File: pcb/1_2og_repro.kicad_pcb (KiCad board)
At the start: 2 copper layers, 347.1 x 119.3 mm, 226 parts, among them J1 Pico EzMate, J2 548190519, J3 RAW, J4 S3B, Q1 2N7002, SW1 MX_SW_solder, SW10 MX_SW_solder, SW11 MX_SW_solder, SW12 MX_SW_solder, SW13 MX_SW_solder, SW14 MX_SW_solder, SW15 MX_SW_solder, SW16 MX_SW_solder, SW17 MX_SW_solder, SW18 MX_SW_solder, SW19 MX_SW_solder, SW2 MX_SW_solder, SW20 MX_SW_solder, SW21 MX_SW_solder, SW22 MX_SW_solder, SW23 MX_SW_solder, SW24 MX_SW_solder, SW25 MX_SW_solder, SW26 MX_SW_solder, SW27 MX_SW_solder, SW28 MX_SW_solder, SW29 MX_SW_solder, SW3 MX_SW_solder, SW30 MX_SW_solder, SW31 MX_SW_solder, SW32 MX_SW_solder, SW33 MX_SW_solder, SW34 MX_SW_solder, SW35 MX_SW_solder, SW36 MX_SW_solder, SW37 MX_SW_solder, SW38 MX_SW_solder, SW39 MX_SW_solder, SW4 MX_SW_solder, SW40 MX_SW_solder, SW41 MX_SW_solder, SW42 MX_SW_solder, SW43 MX_SW_solder, SW44 MX_SW_solder, SW45 MX_SW_solder, SW46 MX_SW_solder, SW47 MX_SW_solder, SW48 MX_SW_solder, SW49 MX_SW_solder, SW5 MX_SW_solder, SW50 MX_SW_solder, SW51 MX_SW_solder, SW52 MX_SW_solder, SW53 MX_SW_solder, SW54 MX_SW_solder, SW55 MX_SW_solder, SW56 MX_SW_solder, SW57 MX_SW_solder, SW58 MX_SW_solder, SW59 MX_SW_solder, SW6 MX_SW_solder, SW60 MX_SW_solder, SW61 MX_SW_solder, SW62 MX_SW_solder, SW63 MX_SW_solder, SW64 MX_SW_solder, SW65 MX_SW_solder, SW66 MX_SW_solder, SW67 MX_SW_solder, SW68 MX_SW_solder, SW69 MX_SW_solder, SW7 MX_SW_solder, SW70 MX_SW_solder, SW71 MX_SW_solder, SW72 MX_SW_solder, SW73 MX_SW_solder, SW74 MX_SW_solder, SW75 MX_SW_solder, SW76 MX_SW_solder, SW77 MX_SW_solder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

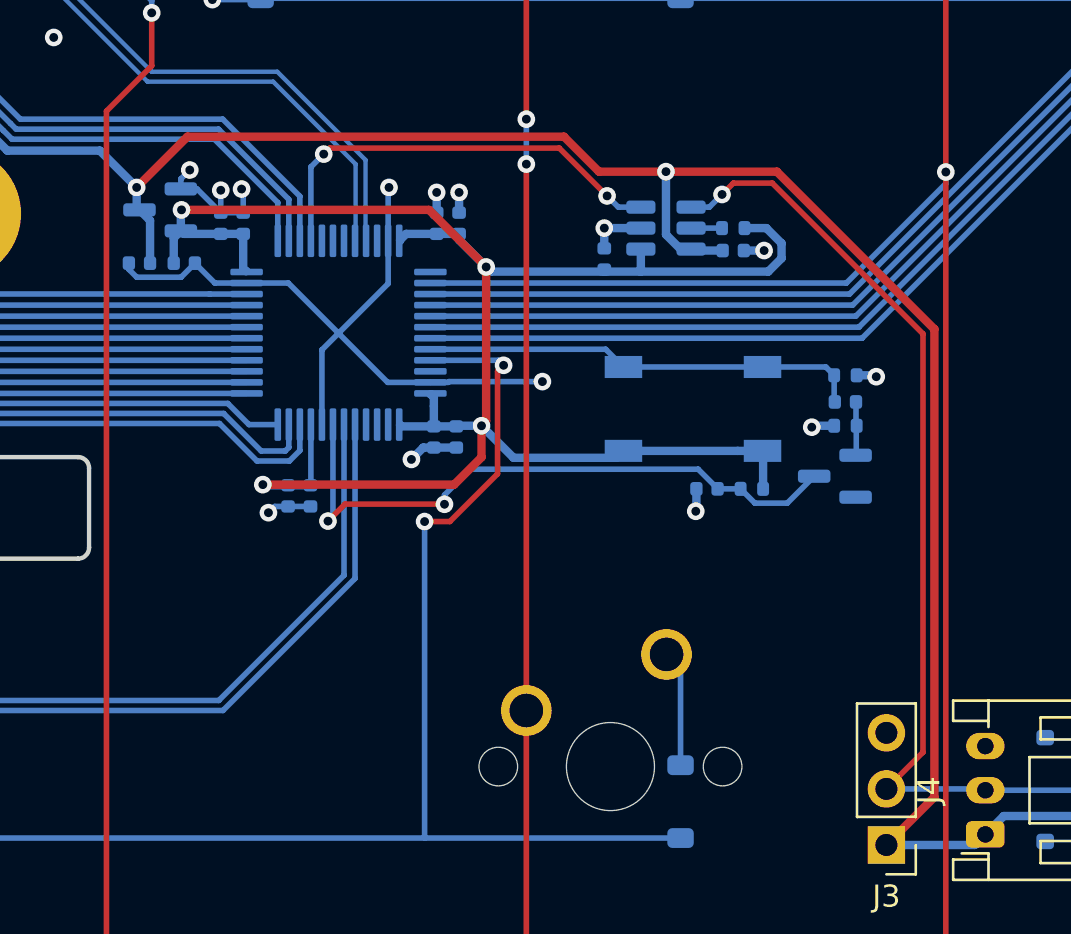
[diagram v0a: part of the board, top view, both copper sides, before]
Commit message: sunday at the waterpark
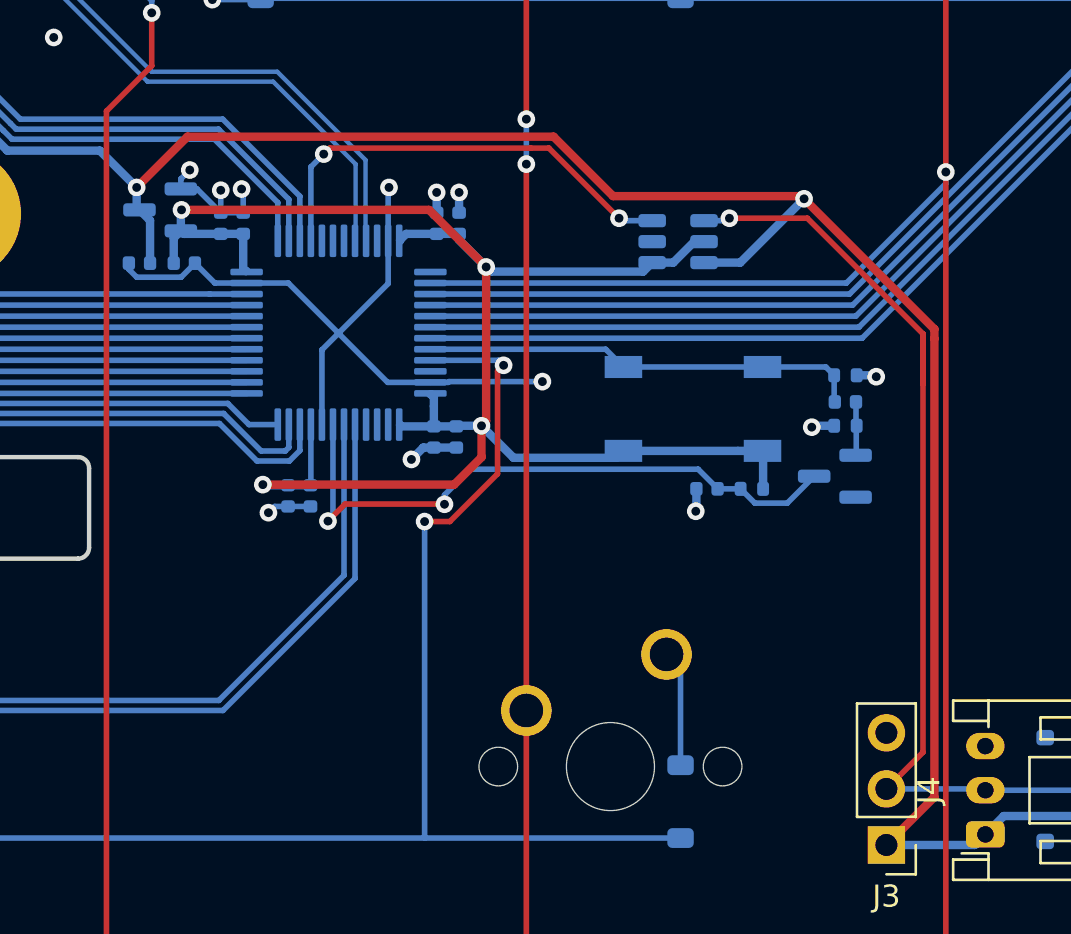
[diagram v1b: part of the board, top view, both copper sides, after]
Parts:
- removed C13, C14: 100nF, Capacitor_SMD:C_0402_1005Metric
- removed R7: 10k, Resistor_SMD:R_0402_1005Metric
- U3: value TXS0101DBV -> SN74LVC1T45DBV; footprint Package_TO_SOT_SMD:SOT-23-6 -> marbastlib-various:SOT-23-6-routable
- moved U3 0.82 mm to (334.2, 84.1)
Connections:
- U3 pad 5: Net-(U3-OE) -> +3V3
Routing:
- net +3V3: track 88.9 -> 82.0 mm
- net GND: track 54.2 -> 50.7 mm, vias 16 -> 14
- net Net-(U3-OE): track 1.40 -> 0.00 mm
- net RGB_3V3: track 19.3 -> 20.1 mm
- net RGBLED: track 46.1 -> 46.7 mm
